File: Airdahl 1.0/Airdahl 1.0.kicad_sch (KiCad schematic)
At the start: 28 parts, among them J1 Conn_ARM_JTAG_SWD_20, SW1 SW_MEC_5E, U1 STM32F446RETx, X2 ABS25-32.768KHZ-6-T, Y1 ABM3B-8.000MHZ-12-D1X-T

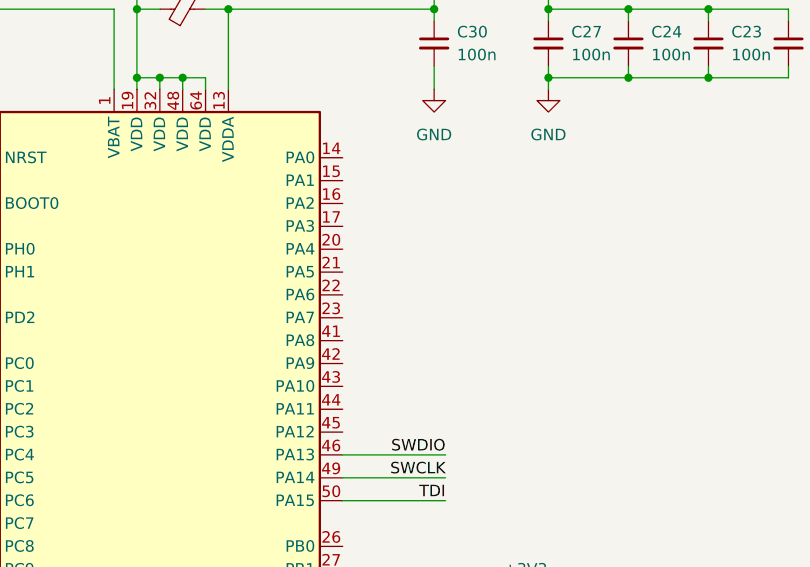
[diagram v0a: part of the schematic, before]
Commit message: rfm wiring
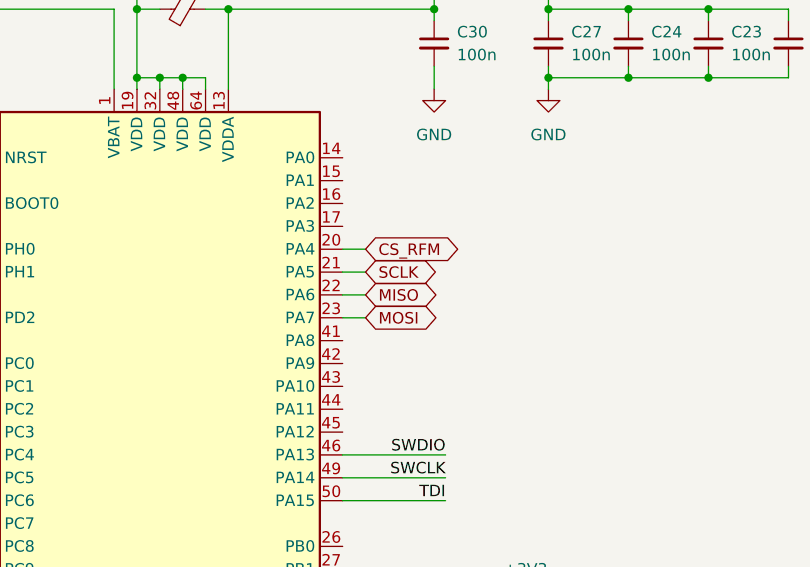
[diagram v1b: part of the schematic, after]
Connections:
- net CS_RFM: now reaches U1.20 (PA4)
- net SCLK: now reaches U1.21 (PA5)
- net MISO: now reaches U1.22 (PA6)
- net MOSI: now reaches U1.23 (PA7)
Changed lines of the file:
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@@
+	(wire
+		(pts
+			(xy 215.9 110.49) (xy 218.44 110.49)
+		)
+		(stroke
+			(width 0)
+			(type default)
+		)
+	)
 	(wire
 		(pts
@@
 	(wire
 		(pts
+			(xy 215.9 107.95) (xy 218.44 107.95)
+		)
+		(stroke
+			(width 0)
+			(type default)
+		)
+	)
+	(wire
+		(pts
 			(xy 135.89 187.96) (xy 135.89 185.42)
 		)
@@
 	(wire
 		(pts
+			(xy 215.9 102.87) (xy 218.44 102.87)
+		)
+		(stroke
+			(width 0)
+			(type default)
+		)
+	)
+	(wire
+		(pts
 			(xy 226.06 82.55) (xy 226.06 85.09)
 		)
@@
 		(pts
 			(xy 135.89 151.13) (xy 144.78 151.13)
+		)
+		(stroke
+			(width 0)
+			(type default)
+		)
+	)
+	(wire
+		(pts
+			(xy 215.9 105.41) (xy 218.44 105.41)
 		)
 		(stroke
@@
 			(effects
 				(font
+					(size 1.27 1.27)
+				)
+				(justify left)
+				(hide yes)
+			)
+		)
+	)
+	(global_label "SCLK"
+		(shape bidirectional)
+		(at 218.44 105.41 0)
+		(fields_autoplaced yes)
+		(effects
+			(font
+				(size 1.27 1.27)
+			)
+			(justify left)
+		)
+		(property "Intersheetrefs" "${INTERSHEET_REFS}"
+			(at 227.3141 105.41 0)
+			(effects
+				(font
+					(size 1.27 1.27)
+				)
+				(justify left)
+				(hide yes)
+			)
+		)
+	)
+	(global_label "CS_RFM"
+		(shape bidirectional)
+		(at 218.44 102.87 0)
+		(fields_autoplaced yes)
+		(effects
+			(font
+				(size 1.27 1.27)
+			)
+			(justify left)
+		)
+		(property "Intersheetrefs" "${INTERSHEET_REFS}"
+			(at 229.7936 102.87 0)
+			(effects
+				(font
+					(size 1.27 1.27)
+				)
+				(justify left)
+				(hide yes)
+			)
+		)
+	)
+	(global_label "MOSI"
+		(shape bidirectional)
+		(at 218.44 110.49 0)
+		(fields_autoplaced yes)
+		(effects
+			(font
+				(size 1.27 1.27)
+			)
+			(justify left)
+		)
+		(property "Intersheetrefs" "${INTERSHEET_REFS}"
+			(at 227.1327 110.49 0)
+			(effects
+				(font
+					(size 1.27 1.27)
+				)
+				(justify left)
+				(hide yes)
+			)
+		)
+	)
+	(global_label "MISO"
+		(shape bidirectional)
+		(at 218.44 107.95 0)
+		(fields_autoplaced yes)
+		(effects
+			(font
+				(size 1.27 1.27)
+			)
+			(justify left)
+		)
+		(property "Intersheetrefs" "${INTERSHEET_REFS}"
+			(at 227.1327 107.95 0)
+			(effects
+				(font
